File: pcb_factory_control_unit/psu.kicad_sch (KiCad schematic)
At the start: 59 parts, among them J4 DC IN, J5 USB STM32, Q1 40N06D, Q2 BSS138, U14 XL6009, U4 TPS54202DDC, U5 TPS54202DDC, U6 MX26631DL, U7 AMS1117-3.3, U8 INA226

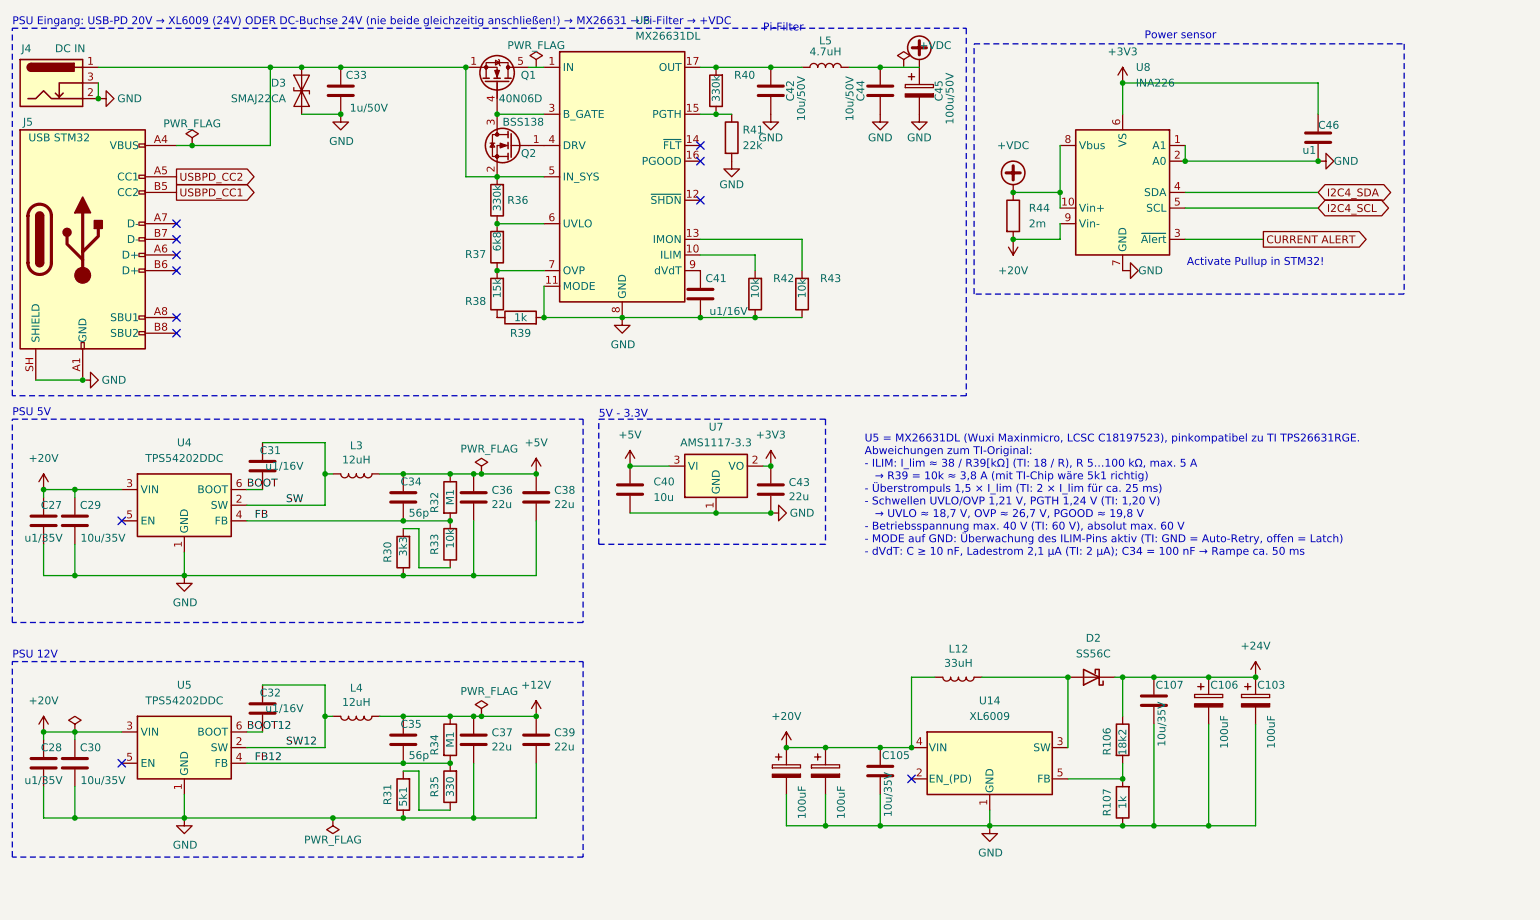
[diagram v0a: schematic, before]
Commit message: New Step Up Controller
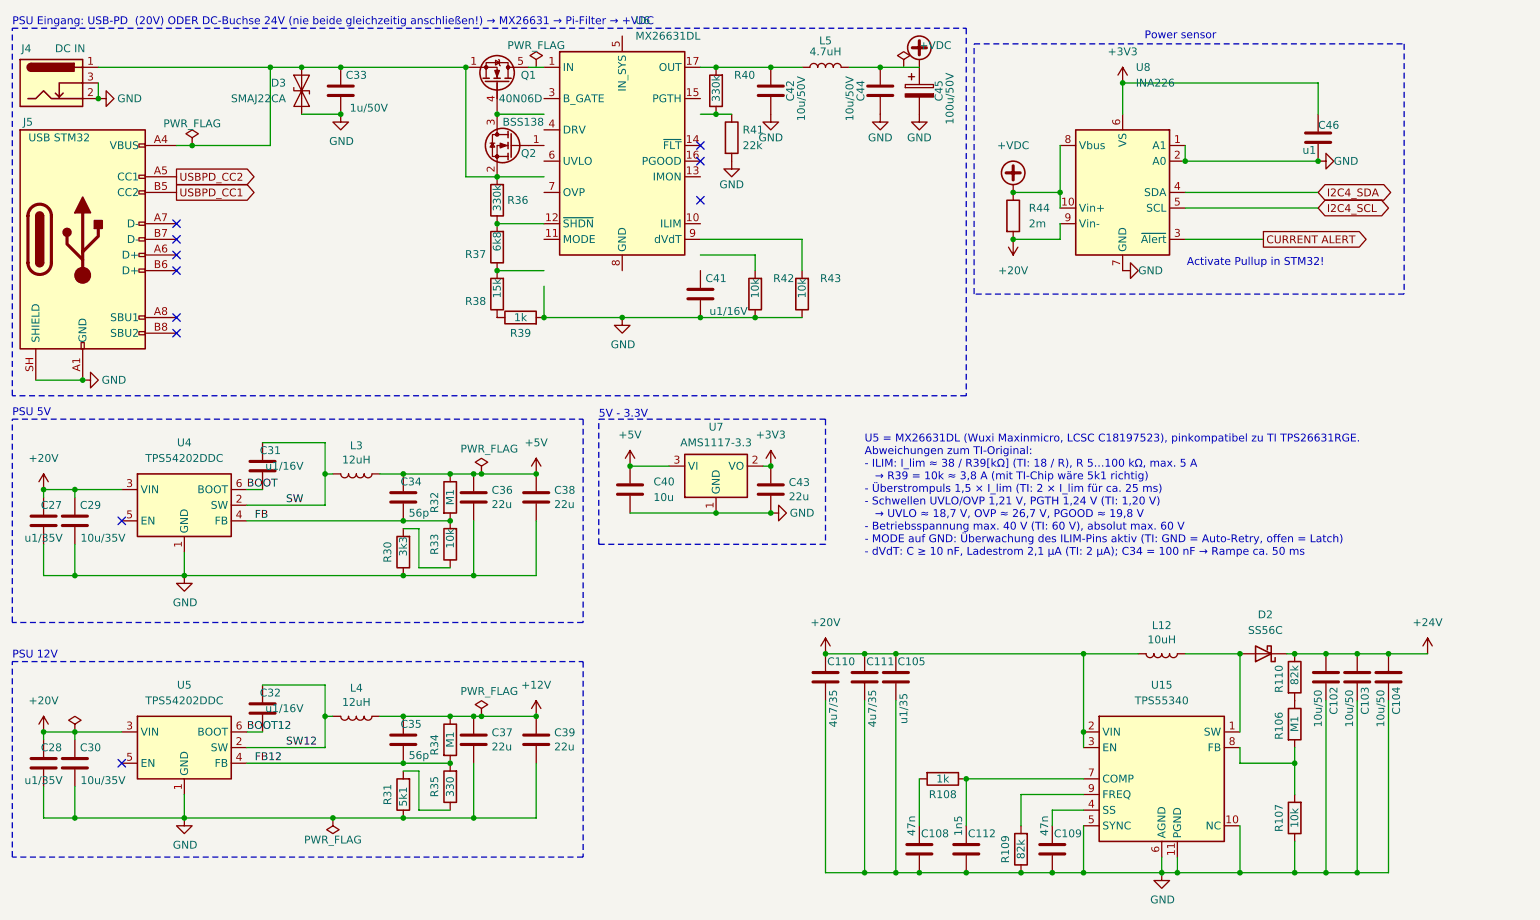
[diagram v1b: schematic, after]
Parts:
- removed C102, C103, C104, C106: 100uF, Capacitor_SMD:CP_Elec_6.3x7.7, symbol Device:C_Polarized
- removed C107: 10u/35V, Capacitor_SMD:C_0805_2012Metric, symbol Device:C
- removed U14: XL6009, Package_TO_SOT_SMD:TO-263-5_TabPin3, symbol liebler_SEMICONDUCTORS:XL6009
- added C102, C103, C104: 10u/50, Capacitor_SMD:C_1210_3225Metric, symbol Device:C
- added C108, C109: 47n, Capacitor_SMD:C_0805_2012Metric, symbol Device:C
- added C110, C111: 4u7/35, Capacitor_SMD:C_0805_2012Metric, symbol Device:C
- added C112: 1n5, Capacitor_SMD:C_0805_2012Metric, symbol Device:C
- added R108: 1k, Resistor_SMD:R_0402_1005Metric, symbol Device:R
- added R109, R110: 82k, Resistor_SMD:R_0402_1005Metric, symbol Device:R
- added U15: TPS55340, Package_DFN_QFN:WQFN-16-1EP_3x3mm_P0.5mm_EP1.68x1.68mm_ThermalVias, symbol liebler_SEMICONDUCTORS:TPS55340
- C105: value 10u/35V -> u1/35
- L12: value 33uH -> 10uH; footprint Inductor_SMD:L_Bourns_SRP1245A -> Inductor_SMD:L_Abracon_ASPI-0630LR; LCSC (none) -> C475521; MPN (none) -> FXL0650-100-M
- R106: value 18k2 -> M1
- R107: value 1k -> 10k
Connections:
- net +20V: now also C110.2, C111.2, U15.2 (VIN), U15.3 (EN)
- net +24V: now also C102.1, C103.1, C104.1, R110.1; no longer R106.1
- net GND: now also C102.2, C103.2, C104.2, C108.1, C109.1, C110.1, C111.1, C112.1, R109.1, U15.10 (NC), U15.11 (PGND), U15.12 (PGND), U15.13 (PGND), U15.14 (NC), U15.17 (AGND), U15.5 (SYNC), U15.6 (AGND); no longer U6.11 (MODE), U6.25 (GND), U6.8 (GND)
- net at R42.2: no longer U6.10 (ILIM)
- net at R40.1, R41.1: no longer U6.15 (PGTH)
- net at C33.2, D3.2 (A2), J4.1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: no longer U6.5 (IN_SYS)
- net at D2.2 (A), L12.1: now also U15.1 (SW), U15.15 (SW), U15.16 (SW)
- net at R37.1, R38.2: no longer U6.7 (OVP)
- net at Q2.1 (G): no longer U6.4 (DRV)
- net at Q1.4 (G), Q2.3 (D): no longer U6.3 (B_GATE)
- net at R106.2, R107.2: now also U15.8 (FB)
- net at R43.2: now also U6.9 (dVdT); no longer U6.13 (IMON)
- net at U6.12 (~{SHDN}): now also R36.1, R37.2
- net at C41.2: no longer U6.9 (dVdT)
- new net: C108.2, R108.2
- new net: R106.1, R110.2
- new net: C112.2, R108.1, U15.7 (COMP)
- new net: R109.2, U15.9 (FREQ)
- new net: C109.2, U15.4 (SS)
- new net: U6.25 (GND), U6.8 (GND)
- now unconnected: U6.6 (UVLO)
- no-connect marks 12 -> 11
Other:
- note added: "PSU Eingang: USB-PD (20V) ODER DC-Buchse 24V (nie beide gleichzeitig anschließen!) → MX26631 → Pi-Filter → +VDC"
- note removed: "PSU Eingang: USB-PD 20V → XL6009 (24V) ODER DC-Buchse 24V (nie beide gleichzeitig anschließen!) → MX26631 → Pi-Filter → +VDC"
- note removed: "Pi-Filter"
- moved on the sheet: C105, D2, L12, R106, R107, U6

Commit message: Step Up Converter
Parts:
- C108, C109, C112: footprint Capacitor_SMD:C_0805_2012Metric -> Capacitor_SMD:C_0402_1005Metric
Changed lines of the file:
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@@
 			)
 		)
-		(property "Footprint" "Capacitor_SMD:C_0805_2012Metric"
+		(property "Footprint" "Capacitor_SMD:C_0402_1005Metric"
 			(at 160.3248 148.59 0)
 			(hide yes)
@@
 			)
 		)
-		(property "Footprint" "Capacitor_SMD:C_0805_2012Metric"
+		(property "Footprint" "Capacitor_SMD:C_0402_1005Metric"
 			(at 167.9448 148.59 0)
 			(hide yes)
@@
 			)
 		)
-		(property "Footprint" "Capacitor_SMD:C_0805_2012Metric"
+		(property "Footprint" "Capacitor_SMD:C_0402_1005Metric"
 			(at 181.9148 148.59 0)
 			(hide yes)
